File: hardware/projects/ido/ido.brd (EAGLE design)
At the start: 49.7 x 49.7 mm, 36 parts, among them U1 PADI-IOT-STAMP, U2 POLOLU-BUCK, U3 AL8805W5, U4 AL8805W5, U5 AL8805W5, X1 PROGRAMMING-HEADER, X10 WIRE-HOLE, X2 UART-HEADER, X3 WIRE-HOLE, X4 WIRE-HOLE, X5 WIRE-HOLE, X6 WIRE-HOLE, X7 WIRE-HOLE, X8 WIRE-HOLE, X9 WIRE-HOLE

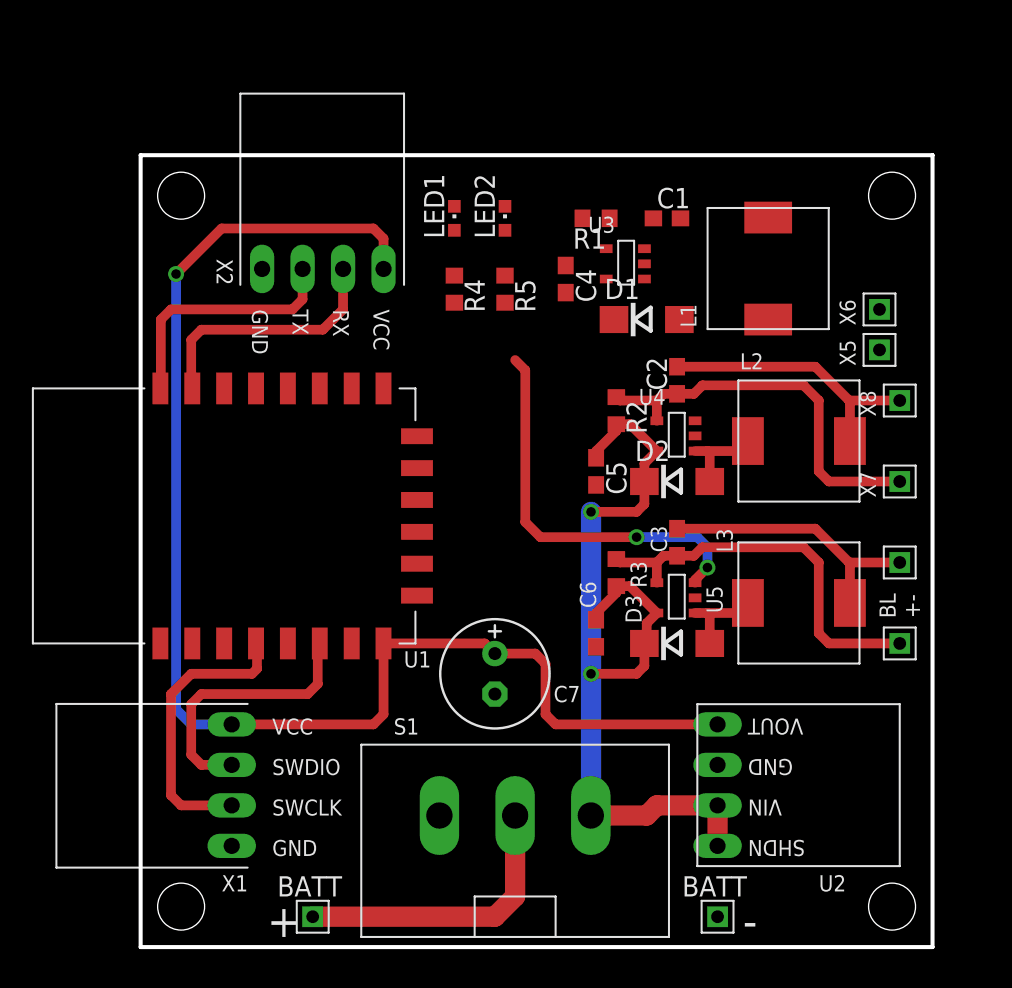
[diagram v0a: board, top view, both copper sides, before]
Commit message: Final board rev.
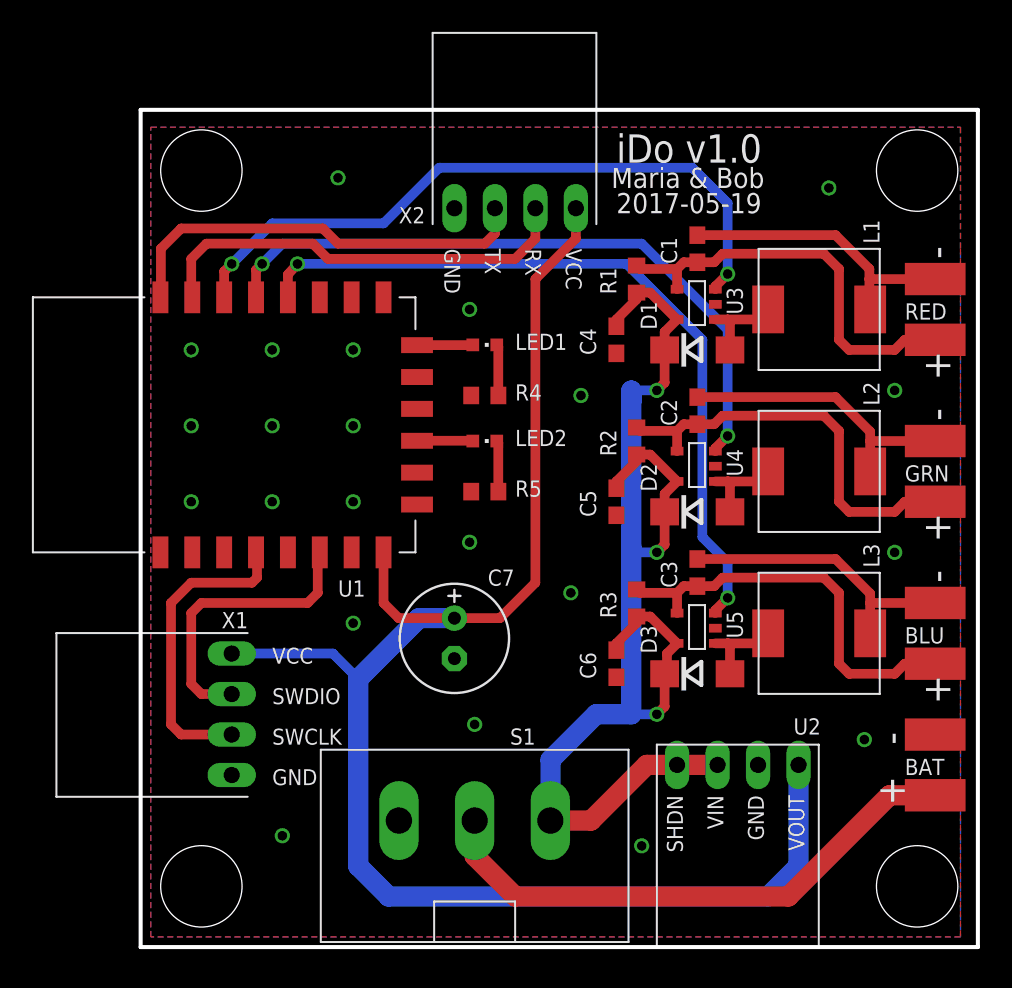
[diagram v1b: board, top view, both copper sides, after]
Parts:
- moved X3 39.8 mm to (49.8, 9.53), turned to 90 degrees
- moved X4 17.8 mm to (49.8, 13.3), turned to 90 degrees
- moved LED2 14.0 mm to (21.6, 31.8), turned to 270 degrees
- moved R5 12.8 mm to (21.6, 28.6), turned to 0 degrees
- moved X2 12.7 mm to (19.7, 46.4)
- moved LED1 8.16 mm to (21.6, 37.8), turned to 270 degrees
- moved R4 6.93 mm to (21.6, 34.6), turned to 0 degrees
- moved U1 5.71 mm to (15.2, 24.8)
- moved U2 5.68 mm to (41.3, 11.4), turned to 180 degrees
- moved U3 5.12 mm to (33.7, 41.3)
- moved C4 4.96 mm to (29.8, 38.1)
- moved R1 4.58 mm to (31.1, 41.9), turned to 270 degrees
- moved X1 4.45 mm to (5.71, 10.8)
- moved X6 3.98 mm to (49.8, 41.9)
- moved D1 3.70 mm to (34.9, 37.5)
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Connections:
- removed net N$2: LED1.A, R4.1
- new net N$5: LED1.C, R4.2
- net DEBUG1: now also LED1.A; no longer R4.2
- net DEBUG2: now also LED2.A; no longer R5.2
- net GND: now also R4.1, R5.1; no longer LED1.C, LED2.C
- net N$3: now also LED2.C, R5.2; no longer LED2.A, R5.1
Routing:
- net RCTRL: track 0.00 -> 42.5 mm, vias 0 -> 2
- net GCTRL: track 0.00 -> 42.2 mm, vias 0 -> 2
- net R+: track 0.00 -> 25.9 mm
- net V+: track 56.0 -> 80.4 mm, vias 2 -> 3
- net BCTRL: track 25.1 -> 47.9 mm
- net R-: track 0.00 -> 18.4 mm
- net N$1: track 18.3 -> 34.8 mm
- net +3V3: track 86.7 -> 102.1 mm, vias 1 -> 0
- net RX: track 15.9 -> 27.3 mm
- net TX: track 15.7 -> 26.8 mm
- net N$4: track 0.00 -> 5.55 mm
- net DEBUG1: track 0.00 -> 3.51 mm
- net DEBUG2: track 0.00 -> 3.51 mm
- net N$3: track 0.00 -> 3.22 mm
- net N$5: track 0.00 -> 3.22 mm
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- added copper zone on layer 1, net GND
- added copper zone on layer 16, net GND
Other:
- board size 49.7 x 49.7 mm -> 52.5 x 52.5 mm
- board text added: "2017-05-19"
- board text added: "BAT"
- board text added: "BLU"
- board text added: "GRN"
- board text added: "Maria & Bob"
- board text added: "RED"
- board text added: "iDo v1.0"
- board text removed: "BATT"
- board text removed: "BL +-"
